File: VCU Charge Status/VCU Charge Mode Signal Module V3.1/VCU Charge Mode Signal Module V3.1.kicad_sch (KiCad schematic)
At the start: 5 parts, among them J1 PH1-10-UA, U1 IRLML2060TRPBF

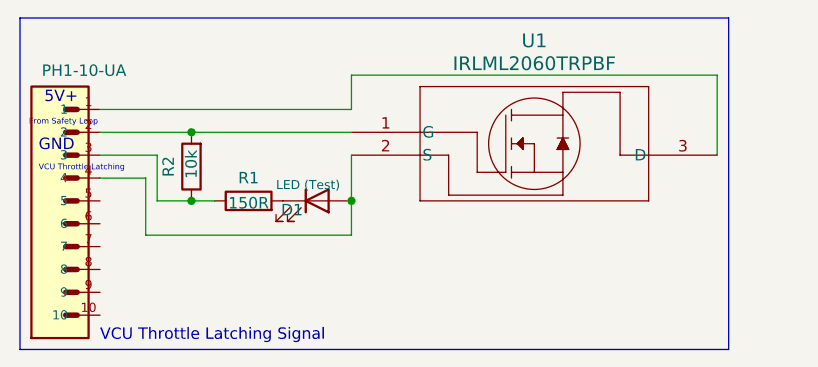
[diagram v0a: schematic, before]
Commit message: More updates
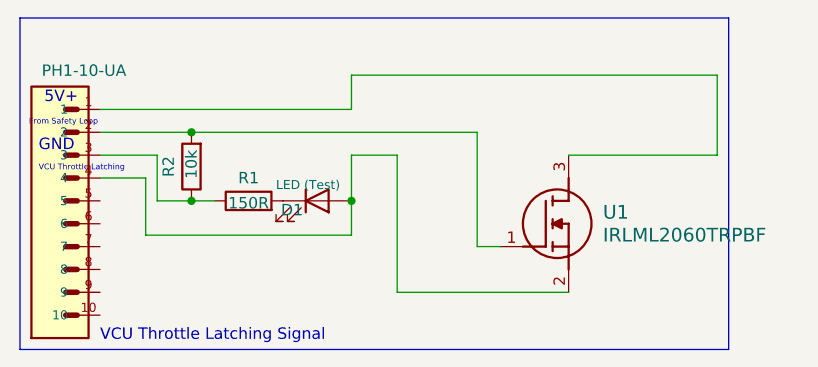
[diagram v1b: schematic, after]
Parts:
- U1: footprint SOT23_INF -> SOT95P237X112-3N; symbol NMOS:IRLML2060TRPBF -> IRLML2060TRPBF:IRLML2060TRPBF; Arrow Part Number (none) -> IRLML2060TRPBF; Arrow Price/Stock (none) -> https://www.arrow.com/en/products/irlml2060trpbf/infineon-t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; Height (none) -> 1.12; Manufacturer_Name (none) -> Infineon; Manufacturer_Part_Number (none) -> IRLML2060TRPBF; Mouser Part Number (none) -> 942-IRLML2060TRPBF; Mouser Price/Stock (none) -> https://www.mouser.co.uk/ProductDetail/Infineon-Technologie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
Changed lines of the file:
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@@
+	(wire
+		(pts
+			(xy 57.15 48.26) (xy 52.07 48.26)
+		)
+		(stroke
+			(width 0)
+			(type default)
+		)
+	)
 	(wire
 		(pts
@@
 	(wire
 		(pts
+			(xy 76.2 48.26) (xy 92.71 48.26)
+		)
+		(stroke
+			(width 0)
+			(type default)
+		)
+	)
+	(wire
+		(pts
+			(xy 76.2 63.5) (xy 57.15 63.5)
+		)
+		(stroke
+			(width 0)
+			(type default)
+		)
+	)
+	(wire
+		(pts
+			(xy 66.04 45.72) (xy 34.29 45.72)
+		)
+		(stroke
+			(width 0)
+			(type default)
+		)
+	)
+	(wire
+		(pts
+			(xy 66.04 58.42) (xy 66.04 45.72)
+		)
+		(stroke
+			(width 0)
+			(type default)
+		)
+	)
+	(wire
+		(pts
 			(xy 30.48 48.26) (xy 24.13 48.26)
 		)
@@
 	(wire
 		(pts
-			(xy 34.29 45.72) (xy 52.07 45.72)
+			(xy 66.04 58.42) (xy 68.58 58.42)
+		)
+		(stroke
+			(width 0)
+			(type default)
+		)
+	)
+	(wire
+		(pts
+			(xy 57.15 63.5) (xy 57.15 48.26)
 		)
 		(stroke
@@
 	)
 	(symbol
-		(lib_id "NMOS:IRLML2060TRPBF")
-		(at 52.07 45.72 0)
+		(lib_id "IRLML2060TRPBF:IRLML2060TRPBF")
+		(at 68.58 58.42 0)
 		(unit 1)
 		(exclude_from_sim no)
@@
 		(fields_autoplaced yes)
 		(property "Reference" "U1"
-			(at 72.39 35.56 0)
+			(at 80.01 54.6099 0)
 			(effects
 				(font
 					(size 1.524 1.524)
 				)
+				(justify left)
 			)
 		)
 		(property "Value" "IRLML2060TRPBF"
-			(at 72.39 38.1 0)
+			(at 80.01 57.1499 0)
 			(effects
 				(font
 					(size 1.524 1.524)
 				)
-			)
-		)
-		(property "Footprint" "SOT23_INF"
-			(at 52.07 45.72 0)
-			(effects
-				(font
-					(size 1.27 1.27)
-					(italic yes)
-				)
-				(hide yes)
-			)
-		)
-		(property "Datasheet" "IRLML2060TRPBF"
-			(at 52.07 45.72 0)
-			(effects
-				(font
-					(size 1.27 1.27)
-					(italic yes)
-				)
-				(hide yes)
-			)
-		)
-		(property "Description" ""
-			(at 52.07 45.72 0)
-			(effects
-				(font
-					(size 1.27 1.27)
-				)
-				(hide yes)
-			)
+				(justify left)
+			)
+		)
+		(property "Footprint" "SOT95P237X112-3N"
+			(at 80.01 157.15 0)
+			(effects
+				(font
+					(size 1.27 1.27)
+				)
+				(justify left top)
+				(hide yes)
+			)
+		)
+		(property "Datasheet" "https://www.infineon.com/dgdl/irlml2060pbf.pdf?fileId=5546d462533600a401535664b7fb25ee"
+			(at 80.01 257.15 0)
+			(effects
+				(font
+					(size 1.27 1.27)
+				)
+				(justify left top)
+				(hide yes)
+			)
+		)
+		(property "Description" "IRLML2060TRPBF N-Channel MOSFET, 1.2 A, 60 V HEXFET, 3-Pin SOT-23 Infineon"
+			(at 68.58 58.42 0)
+			(effects
+				(font
+					(size 1.27 1.27)
+				)
+				(hide yes)
+			)
+		)
+		(property "Height" "1.12"
+			(at 80.01 457.15 0)
+			(effects
+				(font
+					(size 1.27 1.27)
+				)
+				(justify left top)
+				(hide yes)
+			)
+		)
+		(property "Manufacturer_Name" "Infineon"
+			(at 80.01 557.15 0)
+			(effects
+				(font
+					(size 1.27 1.27)
+				)
+				(justify left top)
+				(hide yes)
+			)
+		)
+		(property "Manufacturer_Part_Number" "IRLML2060TRPBF"
+			(at 80.01 657.15 0)
+			(effects
+				(font
+					(size 1.27 1.27)
+				)
+				(justify left top)
+				(hide yes)
+			)
+		)
+		(property "Mouser Part Number" "942-IRLML2060TRPBF"
+			(at 80.01 757.15 0)
+			(effects
+				(font
+					(size 1.27 1.27)
+				)
+				(justify left top)
+				(hide yes)
+			)
+		)
+		(property "Mouser Price/Stock" "https://www.mouser.co.uk/ProductDetail/Infineon-Technologies/IRLML2060TRPBF?qs=9%252BKlkBgLFf1IzIjJ4taDPQ%3D%3D"
+			(at 80.01 857.15 0)
+			(effects
+				(font
+					(size 1.27 1.27)
+				)
+				(justify left top)
+				(hide yes)
+			)
+		)
+		(property "Arrow Part Number" "IRLML2060TRPBF"
+			(at 80.01 957.15 0)
+			(effects
+				(font
+					(size 1.27 1.27)
+				)
+				(justify left top)
+				(hide yes)
+			)
+		)
+		(property "Arrow Price/Stock" "https://www.arrow.com/en/products/irlml2060trpbf/infineon-technologies-ag?utm_currency=USD&region=europe"
+			(at 80.01 1057.15 0)
+			(effects
+				(font
+					(size 1.27 1.27)
+				)
+				(justify left top)
+				(hide yes)
+			)
